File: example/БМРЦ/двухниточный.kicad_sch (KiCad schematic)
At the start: 154 parts

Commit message: Наведен порядок с рамками
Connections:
- net at ДТ23. (П): now also Стрелка15.4; no longer Путь3.
- net at Стрелка15.: now also ДТ23. (П); no longer ДТ22. (П)
- net at ДТ22. (П): now also Путь1.; no longer Стрелка15.
- net at ДТ16. (П): now also Стрелка14.; no longer Стрелка15.
- net at ДТ21. (П): now also Стрелка20.6
- net at ЯП21-25.: now also ДТ10. (П), Соединитель10.2, Стрелка14.2
- net at Стрелка13.: now also ДТ14. (П)
- net at Стрелка14.: now also ДТ10. (П); no longer Стрелка13.
- net at ДТ14. (П): now also Путь2.; no longer Стрелка13.
- net at Стрелка10.: now also ДТ4. (П)
- net at Стрелка10.: now also ДТ8. (П); no longer Стрелка10.
- net at ДТ4. (П): no longer Стрелка10.
- net at ДТ1. (П): now also Путь1.2
- net at ДТ8. (П): now also Стрелка11.; no longer Стрелка10.
- net at ДТ10. (П): now also Соединитель9.2, Стрелка12.2, ЯР11-15.; no longer Стрелка14.
- net at Стрелка17.: now also ДТ13. (П)
- net at ДТ11. (П): now also Стрелка13.6; no longer Стрелка17.
- net at ДТ13. (П): now also Стрелка18.; no longer Стрелка17.
- net at ДТ17. (П): now also Путь4.; no longer Стрелка18.
- net at Стрелка9.: now also ДТ24. (П)
- net at ДТ7. (П): now also Стрелка15.; no longer Стрелка9.
- net at ДТ24. (П): no longer Стрелка9.
- net at ЯРМ29П.: now also ДТ19. (П), Электротяга2.2
- net at ЯПНП.: now also ДТ2. (П), ДТ5. (П)
- net at Стрелка13.: now also Стрелка11.
- net at Стрелка11.: no longer Стрелка13.
- net at ДТ3. (П): now also Соединитель1.2, Стрелка9.2, ЯП1.
- net at Стрелка9.: now also ДТ6. (П); no longer ДТ3. (П)
- net at ДТ6. (П): now also Стрелка12.6, ЯП11-15.; no longer Стрелка9.
- net at ДТ19. (П): now also Стрелка16.4
- net at Стрелка12.: now also Стрелка12.
- net at Стрелка12.: no longer Стрелка12.
- net at Стрелка14.: now also ДТ9. (П); no longer ДТ16. (П)
- net at ЯП9.: now also ДТ9. (П), Стрелка11.6
- net at ДТ15. (П): now also Стрелка16.6
- net at Стрелка19.: now also ДТ18. (П); no longer ДТ15. (П)
- net at Стрелка15.: no longer ДТ7. (П)
- net at ЯП19.: now also ДТ12. (П), Соединитель11.2, Стрелка15.2
- net at ДТ12. (П): now also Стрелка15.
- net at ЯР27.: now also ДТ9. (П), Стрелка14.6
- net at Стрелка11.: now also ДТ5. (П)
- net at ДТ5. (П): no longer Стрелка11.
- net at ДТ18. (П): no longer Стрелка19.
- new net: ДТ23. (П), Путь3.
- new net: ДТ22. (П), Стрелка15. (x2)
- new net: ДТ16. (П), Стрелка15. (x2)
- new net: ДТ23. (П), Стрелка15.
- new net: ДТ22. (П), Стрелка15.5, ЯП35.
- new net: ДТ22. (П), Стрелка15.6, ЯП35.
- new net: ДТ21. (П), Путь6.
- new net: Стрелка13., Стрелка14. (x2)
- new net: ДТ14. (П), Стрелка13.
- new net: ДТ14. (П), Стрелка13.5, ЯР21-25.
- new net: ДТ14. (П), Стрелка13.6, ЯР21-25.
- new net: Стрелка10., Стрелка10. (x2)
- new net: ДТ4. (П), Стрелка10.
- new net: ДТ4. (П), Стрелка10.5, ЯП3-7.
- new net: ДТ4. (П), Стрелка10.6, ЯП3-7.
- new net: ДТ1. (П), ДТ3. (П), ЯРНДП. (x2)
- new net: ДТ8. (П), Стрелка10.
- new net: ДТ10. (П), Стрелка14.
- new net: ДТ4. (П), Изостыки1.1, Тупик1.1, Электротяга1.1, ЯРМ5П.
- new net: ДТ11. (П), Стрелка17. (x2)
- new net: ДТ13. (П), Стрелка17.
- new net: ДТ11. (П), Стрелка17.5, ЯП23.
- new net: ДТ11. (П), Стрелка17.6, ЯП23.
- new net: ДТ17. (П), Стрелка18. (x2)
- new net: ДТ17. (П), Путь4.
- new net: ДТ7. (П), Стрелка9. (x2)
- new net: ДТ24. (П), Стрелка9.
- new net: ДТ19. (П), Электротяга2.1, ЯРМ29П.
- new net: ДТ2. (П), ДТ5. (П), ЯПНП.
- new net: ДТ11. (П), Стрелка13. (x2)
- new net: Стрелка11., Стрелка13.
- new net: ДТ14. (П), Путь2.
- new net: ДТ3. (П), Стрелка9. (x2)
- new net: ДТ6. (П), Стрелка9.
- new net: ДТ6. (П), Стрелка9.5, ЯР1.
- new net: ДТ6. (П), Стрелка9.6, ЯР1.
- new net: ДТ10. (П), Стрелка12. (x2)
- new net: Стрелка12., Стрелка12.
- new net: ДТ20. (П), Электротяга3.1, ЯРМ37П.
- new net: ДТ20. (П), Электротяга3.2, ЯРМ37П.
- new net: ДТ22. (П), Путь1.
- new net: ДТ6. (П), Стрелка12. (x2)
- new net: ДТ6. (П), Стрелка12.5, ЯП11-15.
- new net: ДТ16. (П), Стрелка14.
- new net: ДТ9. (П), Стрелка11.5, ЯП9.
- new net: ДТ15. (П), Стрелка19.5, ЯР33.
- new net: ДТ15. (П), Стрелка19.6, ЯР33.
- new net: ДТ15. (П), Стрелка19. (x2)
- new net: ДТ7. (П), Стрелка15.5, ЯР19.
- new net: ДТ7. (П), Стрелка15.6, ЯР19.
- new net: ДТ7. (П), Стрелка15.
- new net: ДТ12. (П), Стрелка15.
- new net: ДТ9. (П), Стрелка14.5, ЯР27.
- new net: ДТ9. (П), Стрелка11. (x2)
- new net: ДТ5. (П), Стрелка11.
- new net: ДТ9. (П), Стрелка14.
- new net: ДТ18. (П), Стрелка19.
- new net: ДТ8. (П), Стрелка11.
- new net: ДТ13. (П), Стрелка18.
- now unconnected: ДТ18. (П), ДТ2. (П), ДТ2. (П), ДТ20. (П), ДТ20. (П), ДТ24. (П), ДТ4. (П), ДТ4. (П), ДТ4. (П), ДТ4. (П), ДТ5. (П), ДТ5. (П), ДТ5. (П), Стрелка11., Стрелка11., Стрелка11., Стрелка12., Стрелка12., Стрелка12., Стрелка15., Стрелка15., Стрелка15., ЯП1., ЯП11-15., ЯП11-15., ЯП23., ЯП23., ЯП3-7., ЯП3-7., ЯП35., ЯП35., ЯР1., ЯР1., ЯР11-15., ЯР19., ЯР19., ЯР21-25., ЯР21-25., ЯР33., ЯР33., ЯРМ37П., ЯРМ37П., ЯРМ5П., ЯРНДП., ЯРНДП.

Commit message: В двухнитке ЭЦ проложен кабель СЦБ
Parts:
- added К11, К111 (x3), К1111 (x3), К11111, К111111: ~, symbol SCB_Двухнитка:Муфта_ЭЦ
- added Магистральный_1, Магистральный_2, Магистральный_3, Магистральный_4, Магистральный_5, Магистральный_6, Магистральный_7, Магистральный_8, Магистральный_9, Магистральный_кабель1 (x20): ~, symbol SCB:Магистральный_кабель
- added ЭЦ11: ~, symbol SCB:Пост_ЭЦ
- Путь2: Путь IП -> IIП
- ЯП19, ЯП37, ЯР31: Частота1 (none) -> 420/12; Частота2 (none) -> 720/8
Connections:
- net at ДТ23. (П): now also Стрелка15.4; no longer Путь3.
- net at Стрелка15.: now also ДТ23. (П); no longer ДТ22. (П)
- net at ДТ22. (П): now also Путь1.; no longer Стрелка15.
- net at ДТ16. (П): now also Стрелка14.; no longer Стрелка15.
- net at ДТ21. (П): now also Стрелка20.6
- net at Путь6.: no longer ДТ21. (П)
- net at ЯП21-25.: now also ДТ10. (П), Соединитель10.2, Стрелка14.2
- net at Стрелка13.: now also ДТ14. (П)
- net at Стрелка14.: now also ДТ10. (П); no longer Стрелка13.
- net at ДТ14. (П): now also Путь2.; no longer Стрелка13.
- net at Стрелка10.: now also ДТ4. (П)
- net at Стрелка10.: now also ДТ8. (П); no longer Стрелка10.
- net at ДТ4. (П): no longer Стрелка10.
- net at ДТ1. (П): now also Путь1.2
- net at ДТ8. (П): now also Стрелка11.; no longer Стрелка10.
- net at ДТ10. (П): now also Соединитель9.2, Стрелка12.2, ЯР11-15.; no longer Стрелка14.
- net at Стрелка17.: now also ДТ13. (П)
- net at ДТ11. (П): now also Стрелка13.6; no longer Стрелка17.
- net at ДТ13. (П): now also Стрелка18.; no longer Стрелка17.
- net at ДТ17. (П): now also Путь4.; no longer Стрелка18.
- net at Путь4.: no longer ДТ17. (П)
- net at Стрелка9.: now also ДТ24. (П)
- net at ДТ7. (П): now also Стрелка15.; no longer Стрелка9.
- net at ДТ24. (П): no longer Стрелка9.
- net at ЯРМ29П.: now also ДТ19. (П), Электротяга2.2
- net at ЯПНП.: now also ДТ2. (П), ДТ5. (П)
- net at ДТ2. (П), ДТ5. (П): no longer ЯПНП.
- net at Стрелка13.: now also Стрелка11.
- net at Стрелка11.: no longer Стрелка13.
- net at Путь2.: no longer ДТ14. (П)
- net at ДТ3. (П): now also Соединитель1.2, Стрелка9.2, ЯП1.
- net at Стрелка9.: now also ДТ6. (П); no longer ДТ3. (П)
- net at ДТ6. (П): now also Стрелка12.6, ЯП11-15.; no longer Стрелка9.
- net at ДТ19. (П): now also Стрелка16.4
- net at Стрелка12.: now also Стрелка12.
- net at Стрелка12.: no longer Стрелка12.
- net at ЯР31.: now also ДТ13. (П), Стрелка18.
- net at Стрелка14.: now also ДТ9. (П); no longer ДТ16. (П)
- net at ЯП9.: now also ДТ9. (П), Стрелка11.6
- net at ДТ15. (П): now also Стрелка16.6
- net at Стрелка19.: now also ДТ18. (П); no longer ДТ15. (П)
- net at Стрелка15.: no longer ДТ7. (П)
- net at ЯП19.: now also ДТ12. (П), Соединитель11.2, Стрелка15.2
- net at ДТ12. (П): now also Стрелка15.
- net at ЯР27.: now also ДТ9. (П), Стрелка14.6
- net at Стрелка11.: now also ДТ5. (П)
- net at ДТ18. (П): no longer Стрелка19.
- new net: Магистральный_кабель1. (привязка), Магистральный_кабель1. (привязка) (x13)
- new net: ДТ23. (П), Путь3.
- new net: К111., Магистральный_кабель1. (привязка) (x3)
- new net: ДТ22. (П), Стрелка15. (x2)
- new net: ДТ16. (П), Стрелка15. (x2)
- new net: ДТ23. (П), Стрелка15.
- new net: ДТ22. (П), Стрелка15.5, ЯП35.
- new net: ДТ22. (П), Стрелка15.6, ЯП35.
- new net: Магистральный_9. (привязка), Магистральный_кабель1. (привязка)
- new net: Стрелка13., Стрелка14. (x2)
- new net: ДТ14. (П), Стрелка13.
- new net: ДТ14. (П), Стрелка13.5, ЯР21-25.
- new net: ДТ14. (П), Стрелка13.6, ЯР21-25.
- new net: Стрелка10., Стрелка10. (x2)
- new net: ДТ4. (П), Стрелка10.
- new net: ДТ4. (П), Стрелка10.5, ЯП3-7.
- new net: ДТ4. (П), Стрелка10.6, ЯП3-7.
- new net: ДТ1. (П), ДТ3. (П), ЯРНДП. (x2)
- new net: ДТ1. (П), ДТ3. (П) (x2)
- new net: ДТ8. (П), Стрелка10.
- new net: ДТ10. (П), Стрелка14.
- new net: Магистральный_1. (привязка), Магистральный_3. (привязка)
- new net: Магистральный_1. (привязка), Магистральный_кабель1. (привязка)
- new net: ДТ4. (П), Изостыки1.1, Тупик1.1, Электротяга1.1, ЯРМ5П.
- new net: ДТ11. (П), Стрелка17. (x2)
- new net: ДТ13. (П), Стрелка17.
- new net: ДТ11. (П), Стрелка17.5, ЯП23.
- new net: ДТ11. (П), Стрелка17.6, ЯП23.
- new net: ДТ17. (П), Стрелка18. (x2)
- new net: ДТ17. (П), Путь4.
- new net: ДТ7. (П), Стрелка9. (x2)
- new net: ДТ24. (П), Стрелка9.
- new net: ДТ19. (П), Электротяга2.1, ЯРМ29П.
- new net: ДТ2. (П), ДТ5. (П), ЯПНП.
- new net: ДТ11. (П), Стрелка13. (x2)
- new net: Стрелка11., Стрелка13.
- new net: ДТ14. (П), Путь2.
- new net: ДТ3. (П), Стрелка9. (x2)
- new net: ДТ6. (П), Стрелка9.
- new net: ДТ6. (П), Стрелка9.5, ЯР1.
- new net: ДТ6. (П), Стрелка9.6, ЯР1.
- new net: ДТ10. (П), Стрелка12. (x2)
- new net: Стрелка12., Стрелка12.
- new net: К111111., Магистральный_кабель1. (привязка)
- new net: ДТ20. (П), Электротяга3.1, ЯРМ37П.
- new net: ДТ20. (П), Электротяга3.2, ЯРМ37П.
- new net: ДТ22. (П), Путь1.
- new net: К11111., Магистральный_кабель1. (привязка) (x2)
- new net: ДТ6. (П), Стрелка12. (x2)
- new net: ДТ6. (П), Стрелка12.5, ЯП11-15.
- new net: К11., Магистральный_6. (привязка)
- new net: К11., Магистральный_7. (привязка)
- new net: Магистральный_5. (привязка), Магистральный_6. (привязка)
- new net: ДТ16. (П), Стрелка14.
- new net: ДТ9. (П), Стрелка11.5, ЯП9.
- new net: ДТ15. (П), Стрелка19.5, ЯР33.
- new net: ДТ15. (П), Стрелка19.6, ЯР33.
- new net: ДТ15. (П), Стрелка19. (x2)
- new net: ДТ7. (П), Стрелка15.5, ЯР19.
- new net: ДТ7. (П), Стрелка15.6, ЯР19.
- new net: ДТ7. (П), Стрелка15.
- new net: К1111., Магистральный_кабель1. (привязка) (x3)
- new net: К111111., Магистральный_2. (привязка)
- new net: Магистральный_2. (привязка), Магистральный_кабель1. (привязка)
- new net: ДТ12. (П), Стрелка15.
- new net: ДТ9. (П), Стрелка14.5, ЯР27.
- new net: ДТ9. (П), Стрелка11. (x2)
- new net: ДТ5. (П), Стрелка11.
- new net: Магистральный_4. (привязка), Магистральный_5. (привязка)
- new net: ДТ9. (П), Стрелка14.
- new net: ДТ18. (П), Стрелка19.
- new net: ДТ2. (П), ДТ5. (П)
- new net: Магистральный_3. (привязка), Магистральный_4. (привязка)
- new net: ДТ8. (П), Стрелка11.
- new net: Магистральный_8. (привязка), Магистральный_кабель1. (привязка)
- now unconnected: ДТ18. (П), ДТ20. (П), ДТ20. (П), ДТ24. (П), ДТ4. (П), ДТ4. (П), ДТ4. (П), ДТ4. (П), Путь2., Путь4., Путь6., Стрелка11., Стрелка11., Стрелка11., Стрелка12., Стрелка12., Стрелка12., Стрелка15., Стрелка15., Стрелка15., ЯП1., ЯП11-15., ЯП11-15., ЯП23., ЯП23., ЯП3-7., ЯП3-7., ЯП35., ЯП35., ЯР1., ЯР1., ЯР11-15., ЯР19., ЯР19., ЯР21-25., ЯР21-25., ЯР33., ЯР33., ЯРМ37П., ЯРМ37П., ЯРМ5П., ЯРНДП., ЯРНДП.
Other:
- note added: "Ввод каб.СЦБ"

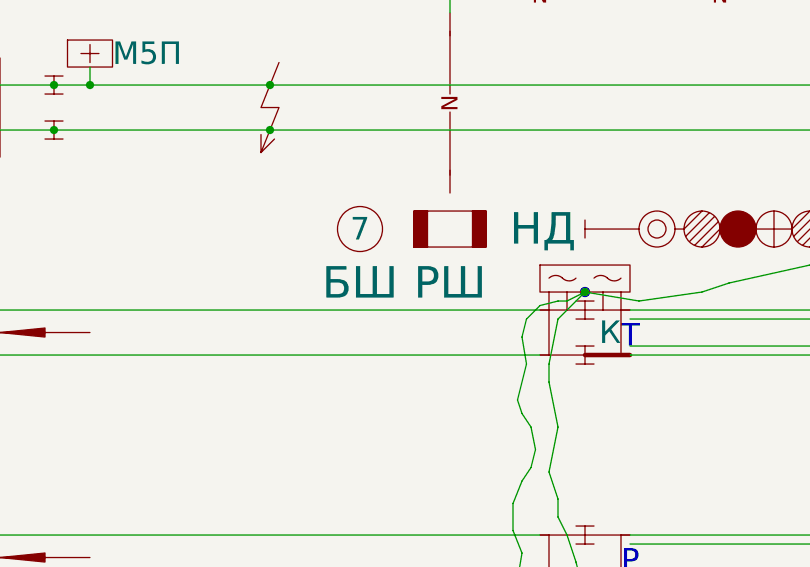
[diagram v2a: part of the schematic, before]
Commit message: Обновлены РШ и БШ
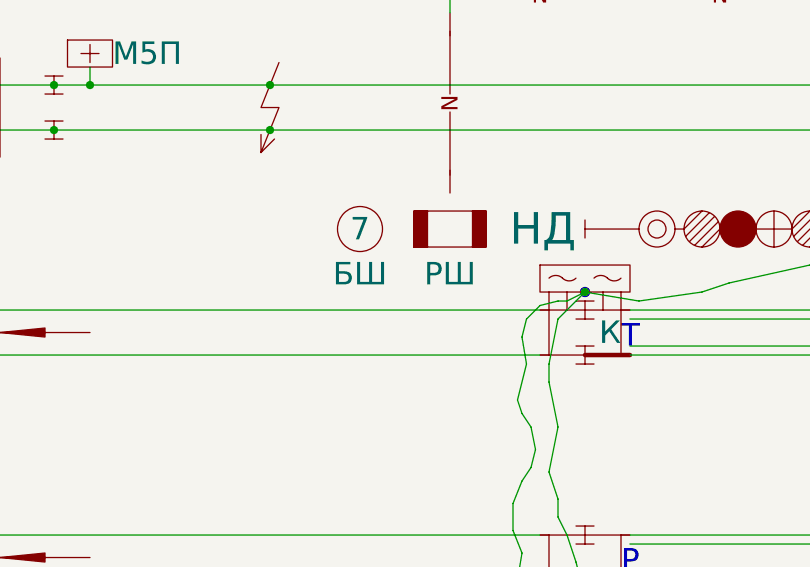
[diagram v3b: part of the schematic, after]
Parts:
- БШ1: Ордината (none) -> (720); Тип (none) -> ШМБ-У
- РШ1: Ордината (none) -> (720); Тип (none) -> ШРУ-М
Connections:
- net at Магистральный_кабель1. (привязка): now also Магистральный_кабель1. (привязка); no longer Магистральный_кабель1. (привязка) (x7)
- net at Магистральный_кабель1. (привязка): now also К111.; no longer Магистральный_кабель1. (привязка)
- net at Путь3.: now also ДТ23. (П)
- net at ДТ23. (П): now also Стрелка15.4; no longer Путь3.
- net at Магистральный_кабель1. (привязка): now also Магистральный_кабель1. (привязка); no longer К111. (x2)
- net at Стрелка15.: now also ДТ23. (П); no longer ДТ22. (П)
- net at ДТ22. (П): now also Путь1.; no longer Стрелка15.
- net at ДТ16. (П): now also Стрелка14.; no longer Стрелка15.
- net at ДТ21. (П): now also Стрелка20.6
- net at Магистральный_кабель1. (привязка): now also Магистральный_кабель1. (привязка); no longer Магистральный_9. (привязка)
- net at ЯП21-25.: now also ДТ10. (П), Соединитель10.2, Стрелка14.2
- net at Стрелка13.: now also ДТ14. (П)
- net at Стрелка14.: now also ДТ10. (П); no longer Стрелка13.
- net at ДТ14. (П): now also Путь2.; no longer Стрелка13.
- net at Стрелка10.: now also ДТ4. (П)
- net at Стрелка10.: now also ДТ8. (П); no longer Стрелка10.
- net at ДТ4. (П): no longer Стрелка10.
- net at ДТ1. (П): now also Путь1.2
- net at ДТ3. (П): now also Соединитель1.2, Стрелка9.2, ЯП1.; no longer ДТ1. (П)
- net at ДТ8. (П): now also Стрелка11.; no longer Стрелка10.
- net at ДТ10. (П): now also Соединитель9.2, Стрелка12.2, ЯР11-15.; no longer Стрелка14.
- net at Магистральный_1. (привязка): now also Магистральный_кабель1. (привязка); no longer Магистральный_3. (привязка)
- net at Магистральный_кабель1. (привязка): now also Магистральный_8. (привязка); no longer Магистральный_1. (привязка)
- net at Стрелка17.: now also ДТ13. (П)
- net at ДТ11. (П): now also Стрелка13.6; no longer Стрелка17.
- net at ДТ13. (П): now also Стрелка18.; no longer Стрелка17.
- net at К111.: now also Магистральный_кабель1. (привязка)
- net at ДТ17. (П): now also Путь4.; no longer Стрелка18.
- net at Путь4.: no longer ДТ17. (П)
- net at Стрелка9.: now also ДТ24. (П)
- net at ДТ7. (П): now also Стрелка15.; no longer Стрелка9.
- net at ДТ24. (П): no longer Стрелка9.
- net at ЯРМ29П.: now also ДТ19. (П), Электротяга2.2
- net at ЯПНП.: now also ДТ2. (П), ДТ5. (П)
- net at ДТ2. (П), ДТ5. (П): no longer ЯПНП.
- net at Стрелка13.: now also Стрелка11.
- net at Стрелка11.: no longer Стрелка13.
- net at Путь2.: no longer ДТ14. (П)
- net at Стрелка9.: now also ДТ6. (П); no longer ДТ3. (П)
- net at ДТ6. (П): now also Стрелка12.6, ЯП11-15.; no longer Стрелка9.
- net at ДТ19. (П): now also Стрелка16.4
- net at Стрелка12.: now also Стрелка12.
- net at Стрелка12.: no longer Стрелка12.
- net at К111111.: no longer Магистральный_кабель1. (привязка)
- net at К11111.: now also Магистральный_кабель1. (привязка)
- net at Магистральный_кабель1. (привязка): now also Магистральный_кабель1. (привязка); no longer К11111.
- net at Магистральный_кабель1. (привязка): now also Магистральный_2. (привязка); no longer К11111.
- net at ЯР31.: now also ДТ13. (П), Стрелка18.
- net at К11.: now also Магистральный_7. (привязка)
- net at Магистральный_6. (привязка): now also Магистральный_5. (привязка); no longer К11.
- net at Магистральный_7. (привязка): no longer К11.
- net at Магистральный_5. (привязка): now also Магистральный_4. (привязка); no longer Магистральный_6. (привязка)
- net at Стрелка14.: now also ДТ9. (П); no longer ДТ16. (П)
- net at Магистральный_кабель1. (привязка): now also К1111.; no longer Магистральный_кабель1. (привязка) (x2)
- net at ЯП9.: now also ДТ9. (П), Стрелка11.6
- net at ДТ15. (П): now also Стрелка16.6
- net at Стрелка19.: now also ДТ18. (П); no longer ДТ15. (П)
- net at Стрелка15.: no longer ДТ7. (П)
- net at К1111.: no longer Магистральный_кабель1. (привязка) (x2)
- net at ЯП19.: now also ДТ12. (П), Соединитель11.2, Стрелка15.2
- net at ДТ12. (П): now also Стрелка15.
- net at ЯР27.: now also ДТ9. (П), Стрелка14.6
- net at Стрелка11.: now also ДТ5. (П)
- net at Магистральный_4. (привязка): now also Магистральный_3. (привязка); no longer Магистральный_5. (привязка)
- net at ДТ18. (П): no longer Стрелка19.
- new net: Магистральный_кабель1. (привязка), Магистральный_кабель1. (привязка) (x2)
- new net: ДТ23. (П), Путь3.
- new net: К111., Магистральный_кабель1. (привязка)
- new net: ДТ22. (П), Стрелка15. (x2)
- new net: ДТ16. (П), Стрелка15. (x2)
- new net: ДТ23. (П), Стрелка15.
- new net: ДТ22. (П), Стрелка15.5, ЯП35.
- new net: ДТ22. (П), Стрелка15.6, ЯП35.
- new net: Магистральный_9. (привязка), Магистральный_кабель1. (привязка)
- new net: Стрелка13., Стрелка14. (x2)
- new net: ДТ14. (П), Стрелка13.
- new net: ДТ14. (П), Стрелка13.5, ЯР21-25.
- new net: ДТ14. (П), Стрелка13.6, ЯР21-25.
- new net: Стрелка10., Стрелка10. (x2)
- new net: ДТ4. (П), Стрелка10.
- new net: ДТ4. (П), Стрелка10.5, ЯП3-7.
- new net: ДТ4. (П), Стрелка10.6, ЯП3-7.
- new net: ДТ1. (П), ДТ3. (П), ЯРНДП. (x2)
- new net: ДТ1. (П), ДТ3. (П) (x2)
- new net: ДТ8. (П), Стрелка10.
- new net: ДТ10. (П), Стрелка14.
- new net: Магистральный_1. (привязка), Магистральный_3. (привязка)
- new net: ДТ4. (П), Изостыки1.1, Тупик1.1, Электротяга1.1, ЯРМ5П.
- new net: ДТ11. (П), Стрелка17. (x2)
- new net: ДТ13. (П), Стрелка17.
- new net: ДТ11. (П), Стрелка17.5, ЯП23.
- new net: ДТ11. (П), Стрелка17.6, ЯП23.
- new net: ДТ17. (П), Стрелка18. (x2)
- new net: ДТ17. (П), Путь4.
- new net: ДТ7. (П), Стрелка9. (x2)
- new net: ДТ24. (П), Стрелка9.
- new net: ДТ19. (П), Электротяга2.1, ЯРМ29П.
- new net: ДТ2. (П), ДТ5. (П), ЯПНП.
- new net: ДТ11. (П), Стрелка13. (x2)
- new net: Стрелка11., Стрелка13.
- new net: ДТ14. (П), Путь2.
- new net: ДТ3. (П), Стрелка9. (x2)
- new net: ДТ6. (П), Стрелка9.
- new net: ДТ6. (П), Стрелка9.5, ЯР1.
- new net: ДТ6. (П), Стрелка9.6, ЯР1.
- new net: ДТ10. (П), Стрелка12. (x2)
- new net: Стрелка12., Стрелка12.
- new net: К111111., Магистральный_кабель1. (привязка)
- new net: ДТ20. (П), Электротяга3.1, ЯРМ37П.
- new net: ДТ20. (П), Электротяга3.2, ЯРМ37П.
- new net: ДТ22. (П), Путь1.
- new net: К11111., Магистральный_кабель1. (привязка)
- new net: ДТ6. (П), Стрелка12. (x2)
- new net: ДТ6. (П), Стрелка12.5, ЯП11-15.
- new net: К11., Магистральный_6. (привязка)
- new net: ДТ16. (П), Стрелка14.
- new net: ДТ9. (П), Стрелка11.5, ЯП9.
- new net: ДТ15. (П), Стрелка19.5, ЯР33.
- new net: ДТ15. (П), Стрелка19.6, ЯР33.
- new net: ДТ15. (П), Стрелка19. (x2)
- new net: ДТ7. (П), Стрелка15.5, ЯР19.
- new net: ДТ7. (П), Стрелка15.6, ЯР19.
- new net: ДТ7. (П), Стрелка15.
- new net: К111111., Магистральный_2. (привязка)
- new net: ДТ12. (П), Стрелка15.
- new net: ДТ9. (П), Стрелка14.5, ЯР27.
- new net: ДТ9. (П), Стрелка11. (x2)
- new net: ДТ5. (П), Стрелка11.
- new net: ДТ9. (П), Стрелка14.
- new net: ДТ18. (П), Стрелка19.
- new net: ДТ2. (П), ДТ5. (П)
- new net: ДТ8. (П), Стрелка11.
- now unconnected: ДТ18. (П), ДТ20. (П), ДТ20. (П), ДТ24. (П), ДТ4. (П), ДТ4. (П), ДТ4. (П), ДТ4. (П), К111111., Путь2., Путь4., Стрелка11., Стрелка11., Стрелка11., Стрелка12., Стрелка12., Стрелка12., Стрелка15., Стрелка15., Стрелка15., ЯП1., ЯП11-15., ЯП11-15., ЯП23., ЯП23., ЯП3-7., ЯП3-7., ЯП35., ЯП35., ЯР1., ЯР1., ЯР11-15., ЯР19., ЯР19., ЯР21-25., ЯР21-25., ЯР33., ЯР33., ЯРМ37П., ЯРМ37П., ЯРМ5П., ЯРНДП., ЯРНДП.
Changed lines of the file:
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@@
 	)
 	(symbol
-		(lib_name "SCB_Двухнитка:Муфта_ЭЦ")
 		(lib_id "SCB_Двухнитка:Муфта_ЭЦ")
 		(at 565 100 0)
@@
 	)
 	(symbol
-		(lib_name "SCB_Двухнитка:Муфта_ЭЦ")
 		(lib_id "SCB_Двухнитка:Муфта_ЭЦ")
 		(at 430 100 0)
@@
 	)
 	(symbol
-		(lib_name "SCB_Двухнитка:Муфта_ЭЦ")
 		(lib_id "SCB_Двухнитка:Муфта_ЭЦ")
 		(at 200 100 0)
@@
 	)
 	(symbol
-		(lib_name "SCB_Двухнитка:Муфта_ЭЦ")
 		(lib_id "SCB_Двухнитка:Муфта_ЭЦ")
 		(at 685 105 0)
@@
 	)
 	(symbol
-		(lib_name "SCB_Двухнитка:Муфта_ЭЦ")
 		(lib_id "SCB_Двухнитка:Муфта_ЭЦ")
 		(at 170 130 0)
@@
 	)
 	(symbol
-		(lib_name "SCB_Двухнитка:Муфта_ЭЦ")
 		(lib_id "SCB_Двухнитка:Муфта_ЭЦ")
 		(at 295 100 0)
@@
 		)
 		(property "Value" "~"
-			(at 85.8 156 0)
+			(at 86.36 156 0)
 			(effects
 				(font
@@
 		)
 		(property "Шкаф" "БШ"
-			(at 90 162 0)
+			(at 90 161 0)
 			(do_not_autoplace yes)
 			(effects
 				(font
-					(size 3.5 3.5)
+					(size 2.5 2.5)
+				)
+			)
+		)
+		(property "Ордината" "(720)"
+			(at 90 151 0)
+			(effects
+				(font
+					(size 2.5 2.5)
 				)
+				(hide yes)
+			)
+		)
+		(property "Тип" "ШМБ-У"
+			(at 90 146 0)
+			(effects
+				(font
+					(size 2.5 2.5)
+				)
+				(hide yes)
 			)
 		)
@@
 		)
 		(property "Шкаф" "РШ"
-			(at 100 162 0)
+			(at 100 161 0)
+			(do_not_autoplace yes)
 			(effects
 				(font
-					(size 3.5 3.5)
+					(size 2.5 2.5)
+				)
+			)
+		)
+		(property "Ордината" "(720)"
+			(at 100 147 0)
+			(effects
+				(font
+					(size 2.5 2.5)
 				)
+				(hide yes)
+			)
+		)
+		(property "Тип" "ШРУ-М"
+			(at 100 151 0)
+			(effects
+				(font
+					(size 2.5 2.5)
+				)
+				(hide yes)
 			)
 		)
@@
 	)
 	(symbol
-		(lib_name "SCB_Двухнитка:Муфта_ЭЦ")
 		(lib_id "SCB_Двухнитка:Муфта_ЭЦ")
 		(at 280 100 0)
@@
 	)
 	(symbol
-		(lib_name "SCB_Двухнитка:Муфта_ЭЦ")
 		(lib_id "SCB_Двухнитка:Муфта_ЭЦ")
 		(at 550 100 0)
@@
 	)
 	(symbol
-		(lib_name "SCB_Двухнитка:Муфта_ЭЦ")
 		(lib_id "SCB_Двухнитка:Муфта_ЭЦ")
 		(at 415 100 0)
